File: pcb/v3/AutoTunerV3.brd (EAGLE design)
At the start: 100 x 80 mm, 113 parts, among them IC2 317EMP, Q1 32,768kHz, Q2 BSS123, Q3 BSS84, U1 TPS63070RNMR, Y1 8MHz

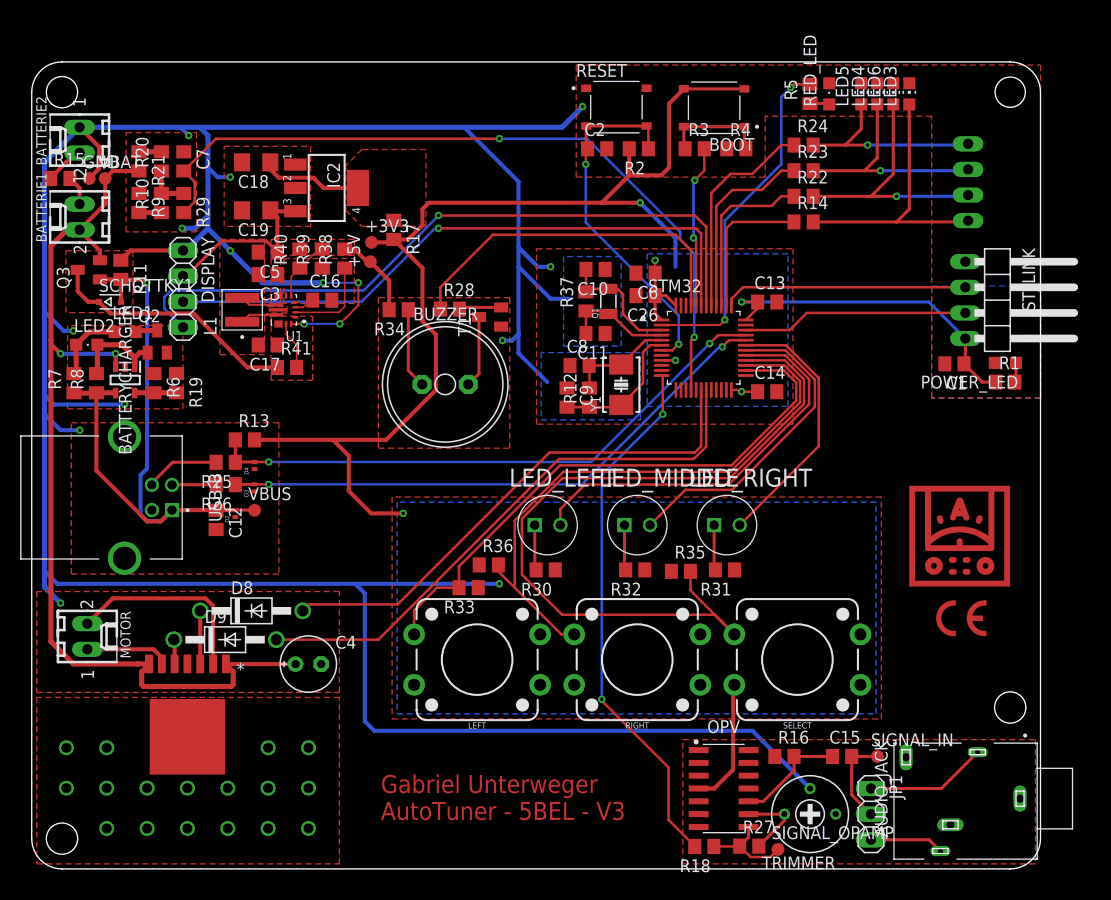
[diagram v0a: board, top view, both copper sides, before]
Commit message: board v3 improvements
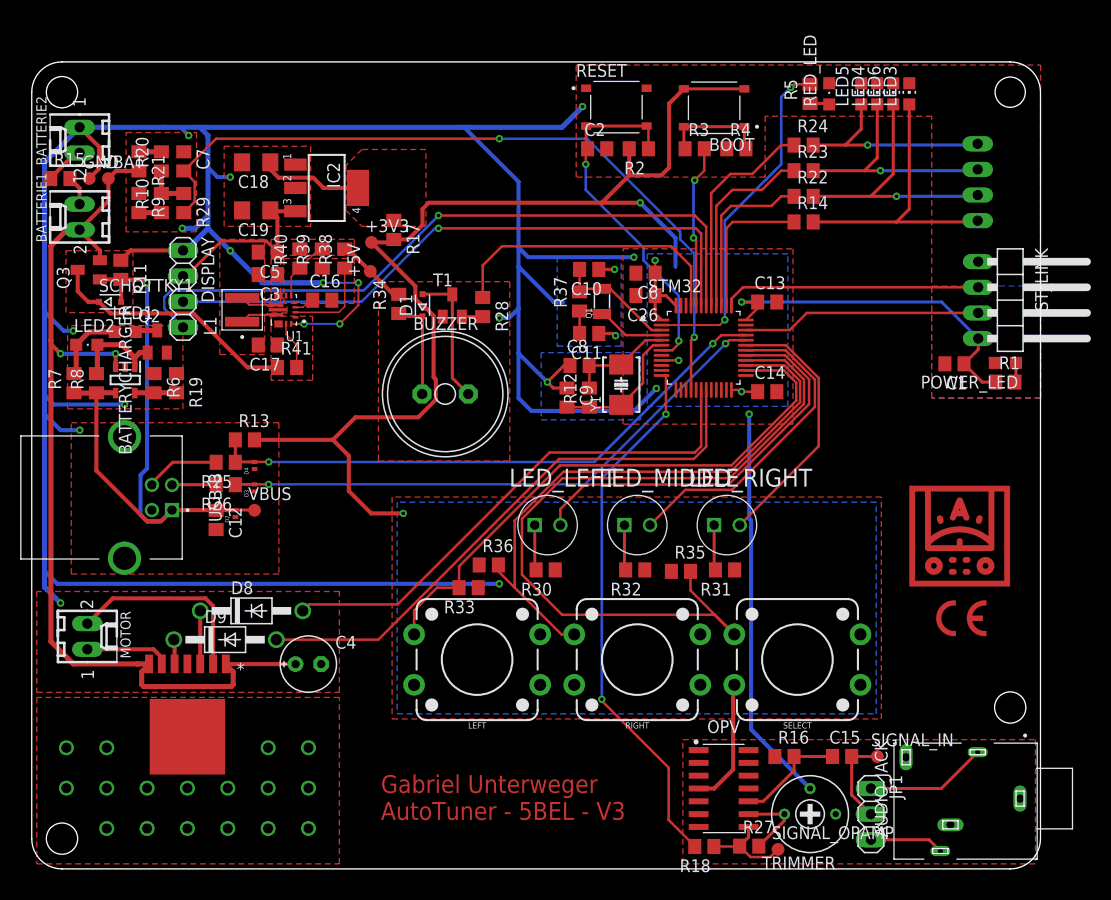
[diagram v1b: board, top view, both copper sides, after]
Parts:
- added D1: (no value), diode:SOD323-R
- R32: value 100 -> 60
- moved T1 3.91 mm to (41.7, 55.8), turned to 0 degrees
- moved R28 3.25 mm to (44.7, 55.7), turned to 270 degrees
- moved ST_LINK 1.27 mm to (97.6, 56.4)
- moved +5V 0.95 mm to (33.6, 59.2)
- moved BUZZER 0.95 mm to (41.0, 47.1)
- moved JP2 0.95 mm to (97.6, 68.1)
- moved C10 0.64 mm to (55.3, 59.4)
- moved C11 0.64 mm to (55.3, 53.1)
- moved R37 0.64 mm to (54.3, 56.3)
- moved Q1 0.63 mm to (56.5, 56.3)
- moved R34 0.58 mm to (36.4, 56.0), turned to 90 degrees
- moved VBAT 0.32 mm to (7.60, 68.4)
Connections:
- net N$54: now also D1.A
- net N$55: now also D1.C
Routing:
- net GND: track 325.5 -> 340.0 mm, vias 16 -> 21
- net N$54: track 7.12 -> 13.5 mm
- net BUZZER: track 35.3 -> 29.3 mm
- net +3V3: track 170.2 -> 173.7 mm
- net N$55: track 7.98 -> 10.2 mm
- net N$56: track 4.19 -> 2.06 mm
- net +5V: track 26.8 -> 25.4 mm
- net SWDIO: track 22.5 -> 23.7 mm
- net SWDCLK: track 24.3 -> 25.6 mm
- net N$50: track 20.1 -> 21.0 mm
- net N$49: track 22.5 -> 23.5 mm
- net N$48: track 25.4 -> 26.4 mm
- net N$39: track 27.6 -> 28.5 mm
- net OSC32OUT: track 10.7 -> 11.3 mm
- net OSC32IN: track 12.7 -> 12.2 mm
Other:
- board text added: "+ -"
- board text added: "+3V3"
- board text added: "+5V"
- board text added: "BuildInLED"
- board text added: "Extenions"
- board text added: "GND"
- board text added: "Input"
- board text added: "SIGNAL_IN"
- board text added: "SIGNAL_OPAMP"
- board text added: "VBAT"
- board text added: "VBUS"
- board text added: "microcontroller"
- board text removed: "-"
- board text removed: "A_IN"
- board text removed: "PC13"
- board text removed: "uC"
